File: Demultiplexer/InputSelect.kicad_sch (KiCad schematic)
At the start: 23 parts, among them SW201 SW_Push_Dual, SW202 SW_Push_Dual, U201 74HC14, U202 74HC74

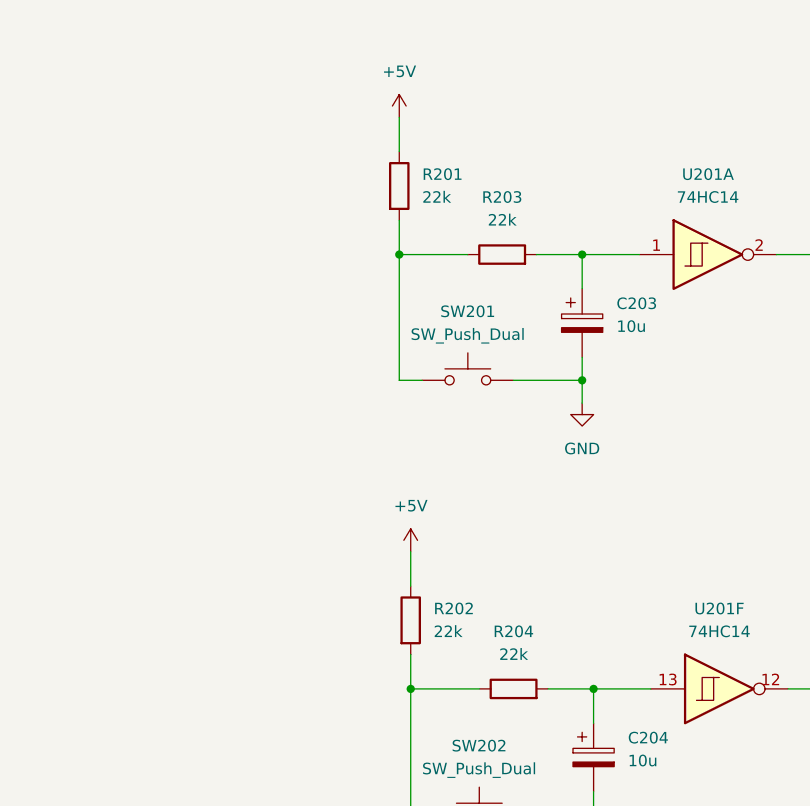
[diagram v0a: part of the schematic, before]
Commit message: Finish roughing out board
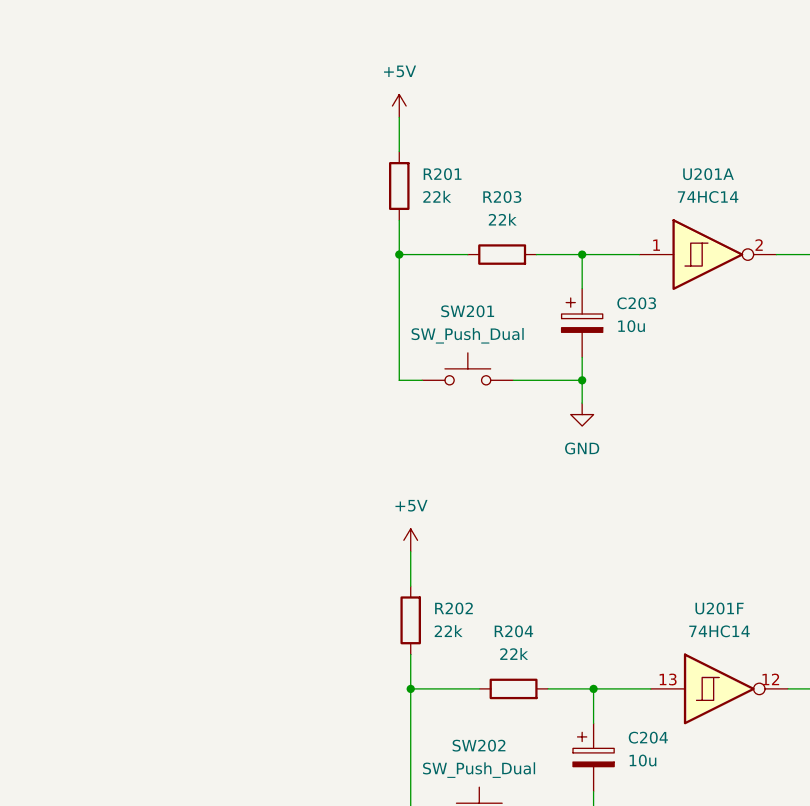
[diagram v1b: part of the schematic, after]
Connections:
- net +5V: now also R201.2, R202.2; no longer R201.1, R202.1
- net at R203.1, SW201.1: now also R201.1; no longer R201.2
- net at R204.1, SW202.1: now also R202.1; no longer R202.2
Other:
- moved on the sheet: R201, R202
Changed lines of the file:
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@@
     (pin "1")
   )
-  (symbol (lib_id "Device:R") (at 88.9 99.06 0) (unit 1)
+  (symbol (lib_id "Device:R") (at 88.9 99.06 180) (unit 1)
     (in_bom yes) (on_board yes) (fields_autoplaced)
     (property "Reference" "R202" (id 0) (at 91.44 97.7899 0)
-      (effects (font (size 1.27 1.27)) (justify left))
+      (effects (font (size 1.27 1.27)) (justify right))
     )
     (property "Value" "22k" (id 1) (at 91.44 100.3299 0)
-      (effects (font (size 1.27 1.27)) (justify left))
+      (effects (font (size 1.27 1.27)) (justify right))
     )
-    (property "Footprint" "Resistor_THT:R_Axial_DIN0207_L6.3mm_D2.5mm_P7.62mm_Horizontal" (id 2) (at 87.122 99.06 90)
+    (property "Footprint" "Resistor_THT:R_Axial_DIN0207_L6.3mm_D2.5mm_P7.62mm_Horizontal" (id 2) (at 90.678 99.06 90)
       (effects (font (size 1.27 1.27)) hide)
     )
@@
     (pin "2")
   )
-  (symbol (lib_id "Device:R") (at 87.63 50.8 0) (unit 1)
+  (symbol (lib_id "Device:R") (at 87.63 50.8 180) (unit 1)
     (in_bom yes) (on_board yes) (fields_autoplaced)
     (property "Reference" "R201" (id 0) (at 90.17 49.5299 0)
-      (effects (font (size 1.27 1.27)) (justify left))
+      (effects (font (size 1.27 1.27)) (justify right))
     )
     (property "Value" "22k" (id 1) (at 90.17 52.0699 0)
-      (effects (font (size 1.27 1.27)) (justify left))
+      (effects (font (size 1.27 1.27)) (justify right))
     )
-    (property "Footprint" "Resistor_THT:R_Axial_DIN0207_L6.3mm_D2.5mm_P7.62mm_Horizontal" (id 2) (at 85.852 50.8 90)
+    (property "Footprint" "Resistor_THT:R_Axial_DIN0207_L6.3mm_D2.5mm_P7.62mm_Horizontal" (id 2) (at 89.408 50.8 90)
       (effects (font (size 1.27 1.27)) hide)
     )
